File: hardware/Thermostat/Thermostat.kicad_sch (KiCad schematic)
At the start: 54 parts, among them J1 Barrel_Jack_Switch, J2 Screw_Terminal_01x02, J3 AVR-ISP-6, J4 MainConnectorr, K1 G6E, K2 G6E, K3 G6E, K4 G6E, SW1 12MM, SW2 12MM, SW3 12MM, SW4 DIP-1, SW5 SW_Push, U1 GU112X16G-7003BL, U4 UA78M05QDCYRQ1, U5 ATmega88-20A, U6 TMP116xxDRV, U7 THVD1500, U8 DS1307Z+, Y1 Crystal, Y2 Crystal_GND23

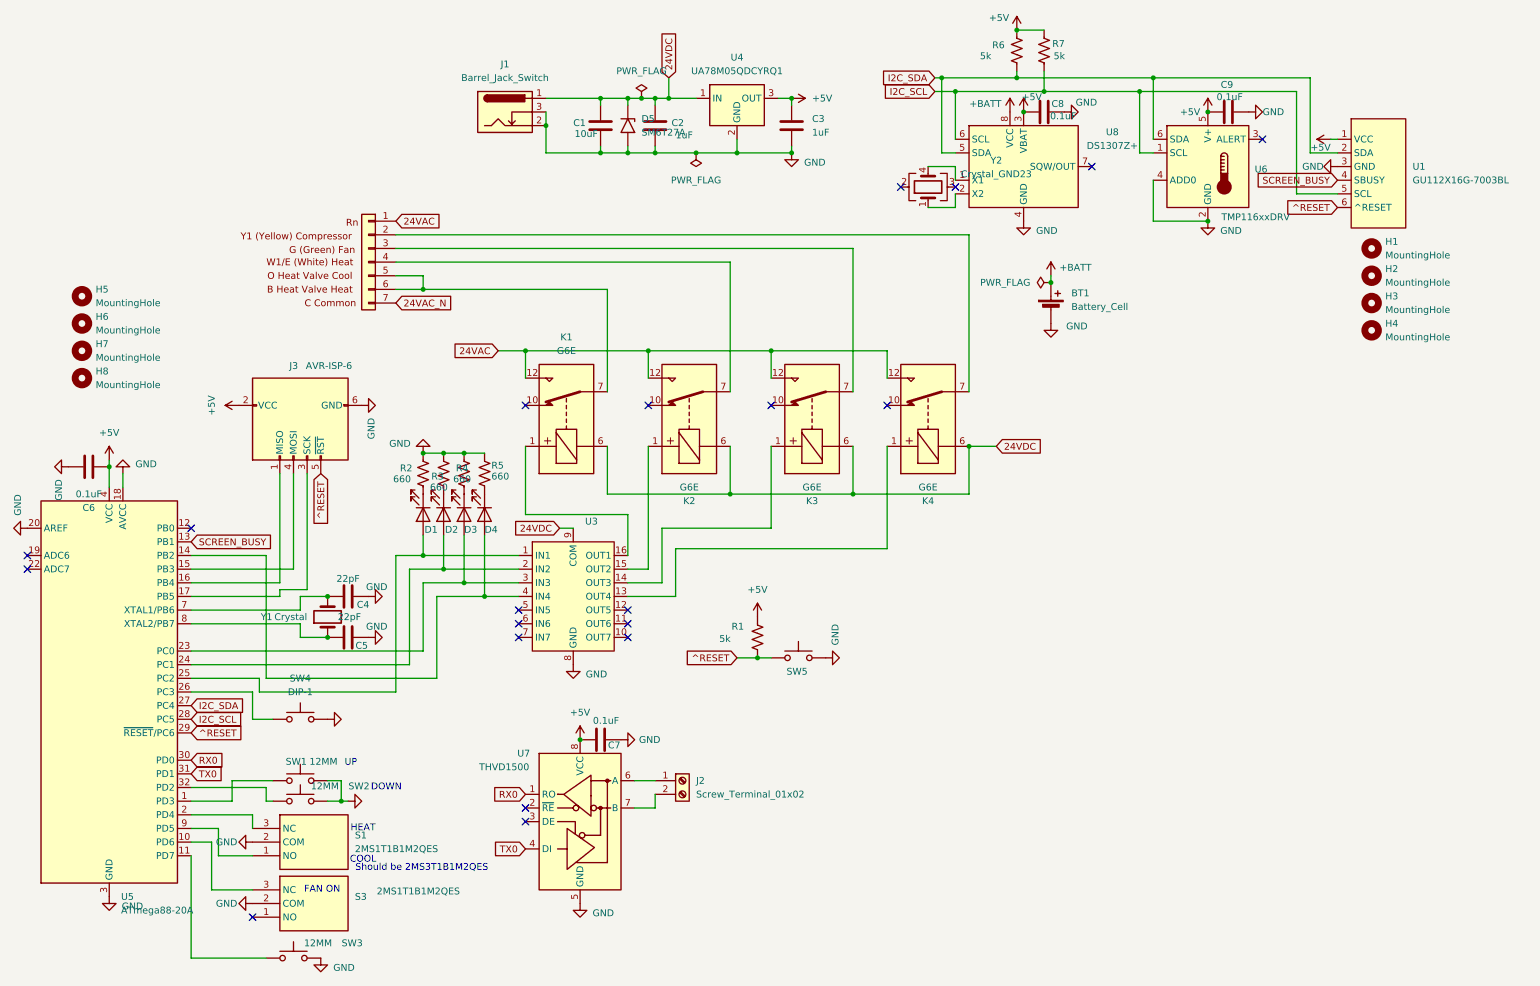
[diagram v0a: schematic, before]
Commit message: WIP
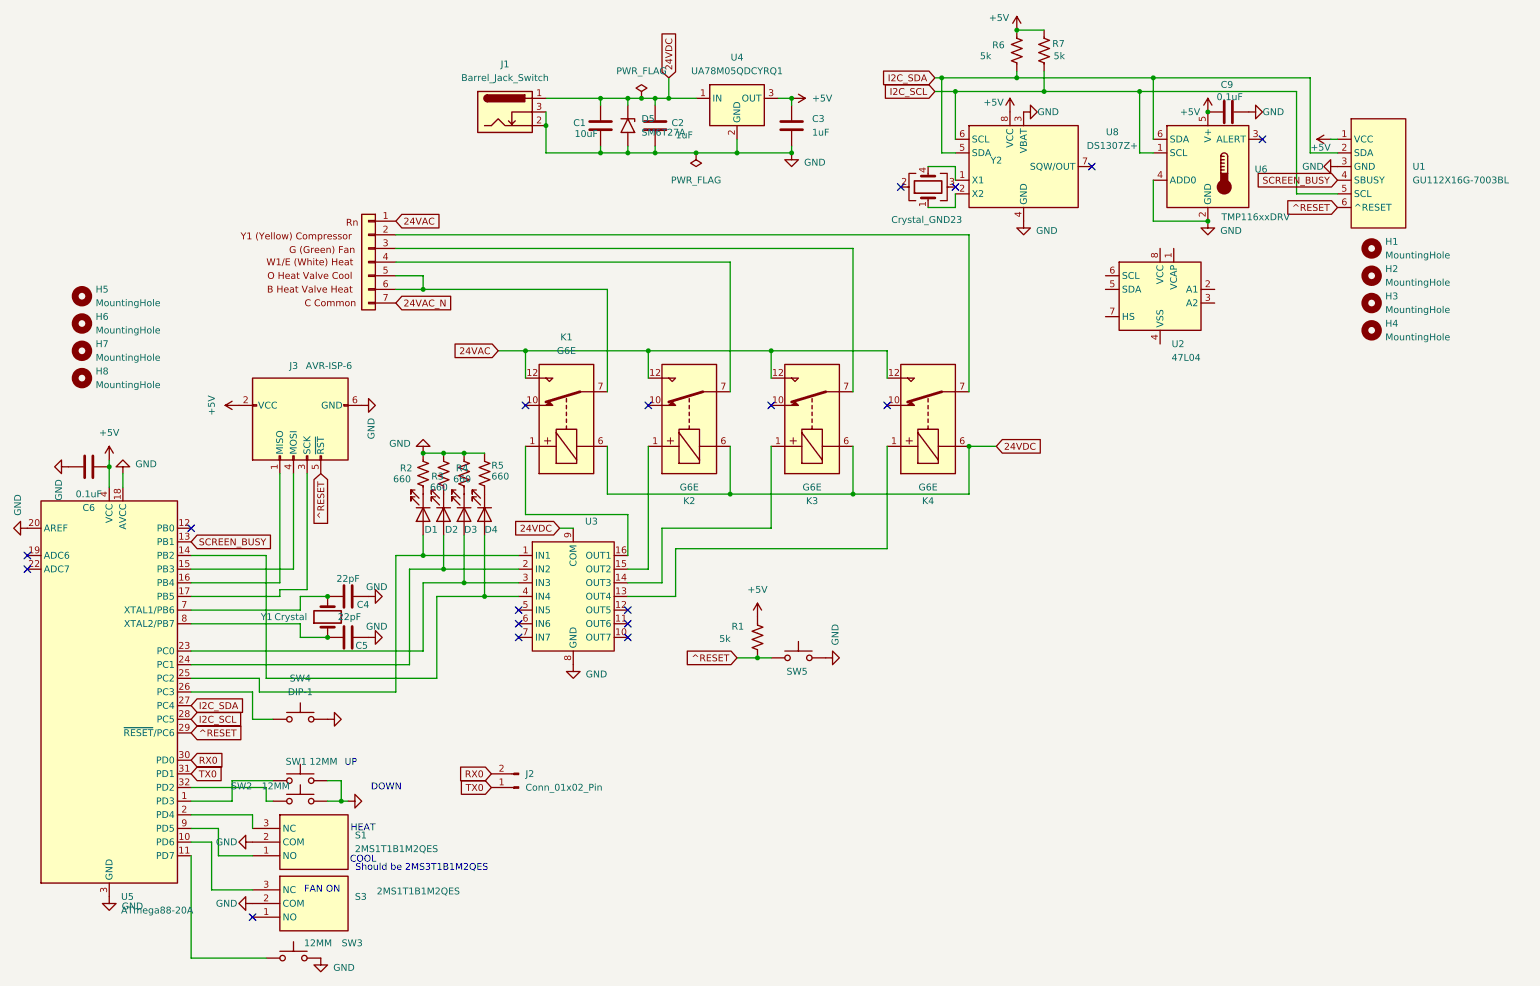
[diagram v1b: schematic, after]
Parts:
- removed BT1: Battery_Cell, Battery:BatteryHolder_Keystone_1058_1x2032, symbol Device:Battery_Cell
- removed C7, C8: 0.1uF, Capacitor_SMD:C_0603_1608Metric, symbol Device:C
- removed J2: Screw_Terminal_01x02, TerminalBlock_MetzConnect:TerminalBlock_MetzConnect_Type094_RT03502HBLU_1x02_P5.00mm_Horizontal, symbol Connector:Screw_Terminal_01x02
- removed U7: THVD1500, Package_SO:SOIC-8_3.9x4.9mm_P1.27mm, symbol Interface_UART:THVD1500
- added J2: Conn_01x02_Pin, Connector_PinHeader_2.54mm:PinHeader_1x02_P2.54mm_Vertical_SMD_Pin1Left, symbol Connector:Conn_01x02_Pin
- added U2: 47L04, Package_SO:SOIC-8_3.9x4.9mm_P1.27mm, symbol Memory_NVRAM:47L04
- Y1: footprint Crystal:Crystal_SMD_HC49-SD -> Crystal:Crystal_SMD_5032-2Pin_5.0x3.2mm
- Y2: footprint ThermostatFootprints:MC-306_EPS -> Crystal:Crystal_SMD_5032-2Pin_5.0x3.2mm
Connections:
- net +BATT is gone; now on net +5V: U8.8 (VCC)
- net +5V: no longer U8.3 (VBAT)
- net GND: now also SW2.1, U8.3 (VBAT); no longer SW2.2
- net RX0: now also J2.2 (Pin_2)
- net TX0: now also J2.1 (Pin_1)
- net at U5.32 (PD2): now also SW2.2; no longer SW2.1
- no-connect marks 20 -> 18
